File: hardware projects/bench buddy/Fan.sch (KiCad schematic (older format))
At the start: 0 parts

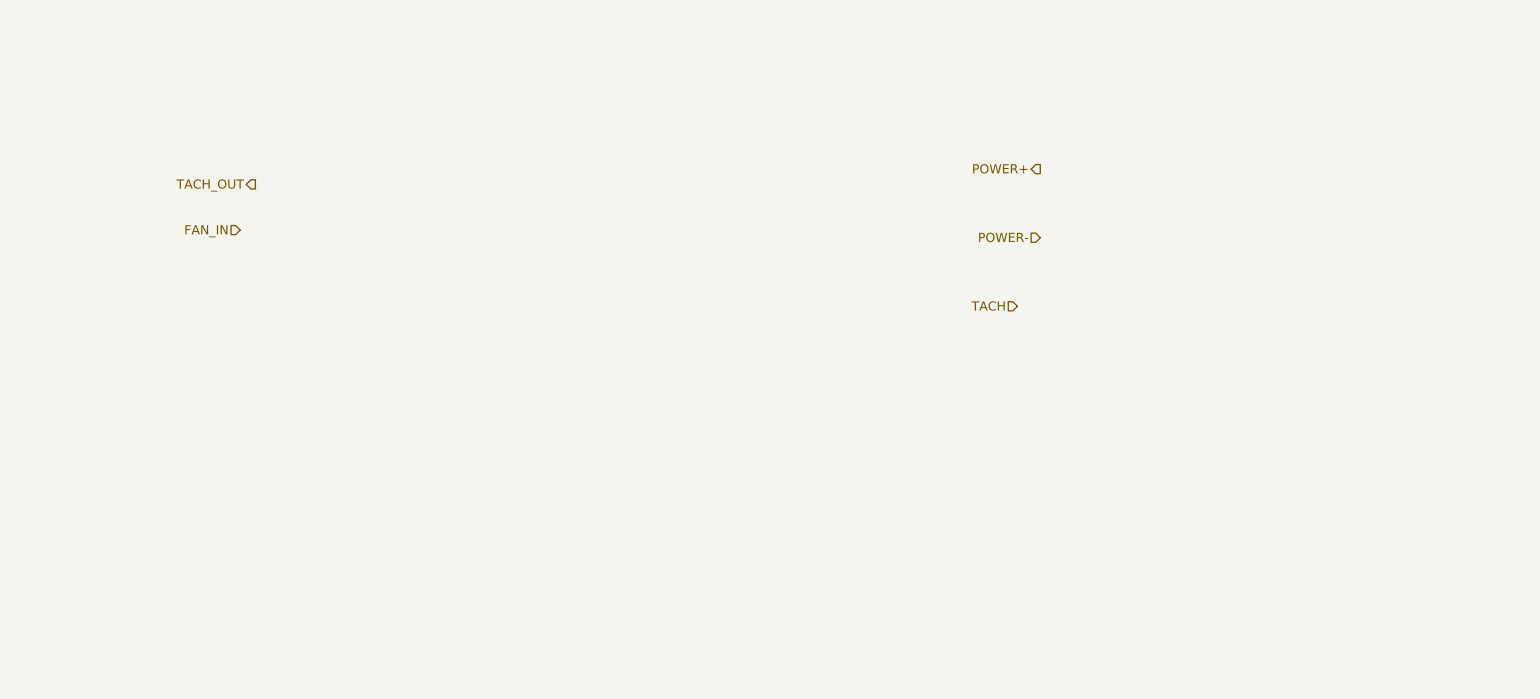
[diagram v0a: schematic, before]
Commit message: FAN DRIVER
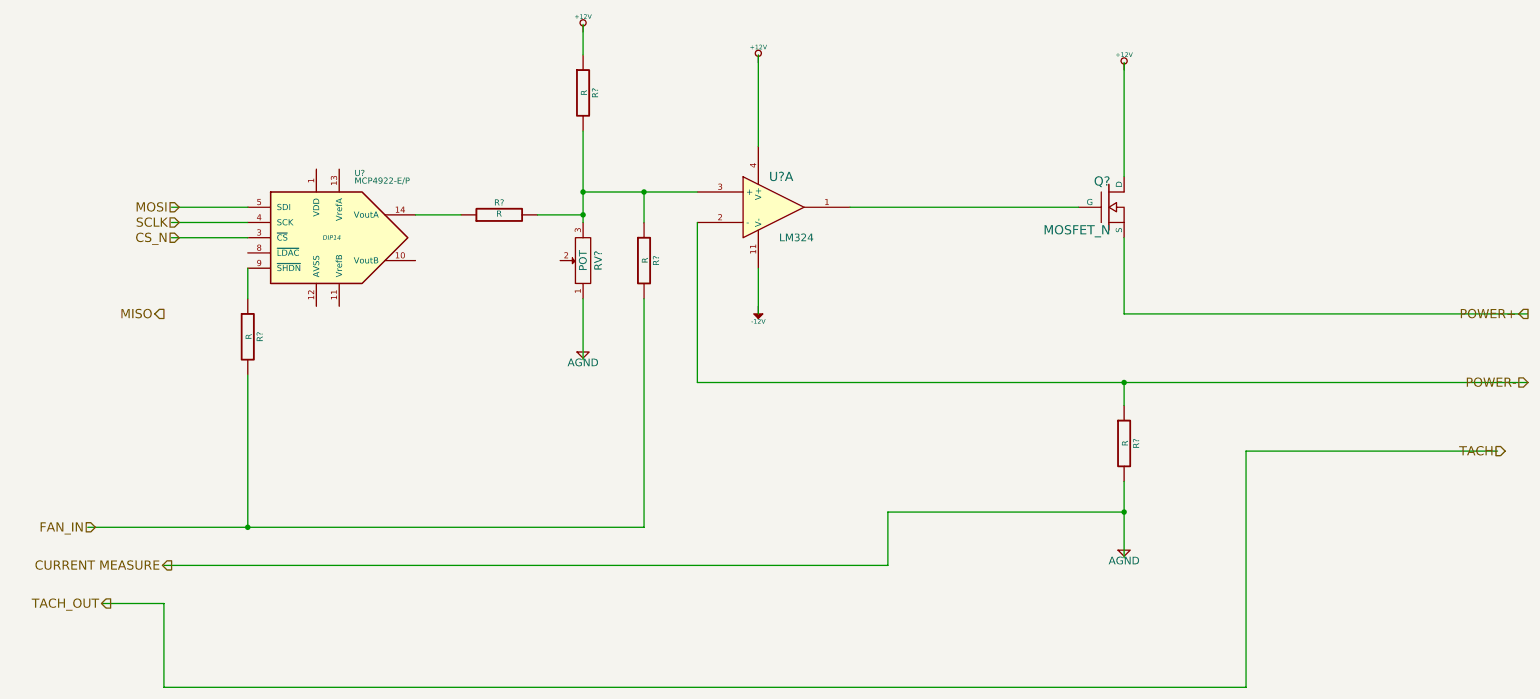
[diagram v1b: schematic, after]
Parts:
- added Q?: MOSFET_N, ~, symbol MOSFET_N
- added R? (x5): R, ~, symbol R
- added RV?: POT, ~, symbol POT
- added U?: LM324, symbol LM324
- added U?: MCP4922-E/P, DIP14, symbol MCP4922-E/P
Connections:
- net labels added: +12V, -12V, AGND, CS_N, CURRENT MEASURE, MISO, MOSI, SCLK
- wire segments 0 -> 32
